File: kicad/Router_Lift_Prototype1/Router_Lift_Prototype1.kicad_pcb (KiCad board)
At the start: 2 copper layers, 150 x 100 mm, 31 parts, among them J1 Conn_01x02, J10 Conn_01x02, J11 Conn_01x04, J2 Conn_01x02, J3 Conn_01x06, J4 Conn_01x06, J5 Conn_01x06, J6 Conn_01x02, J7 Conn_01x02, J8 Conn_01x02, J9 Conn_01x02, Q1 2N7000, Q2 2N7000, U1 SH1106_Display_Module, U2 ESP32-WROOM, U3 BOOST-DRV8711

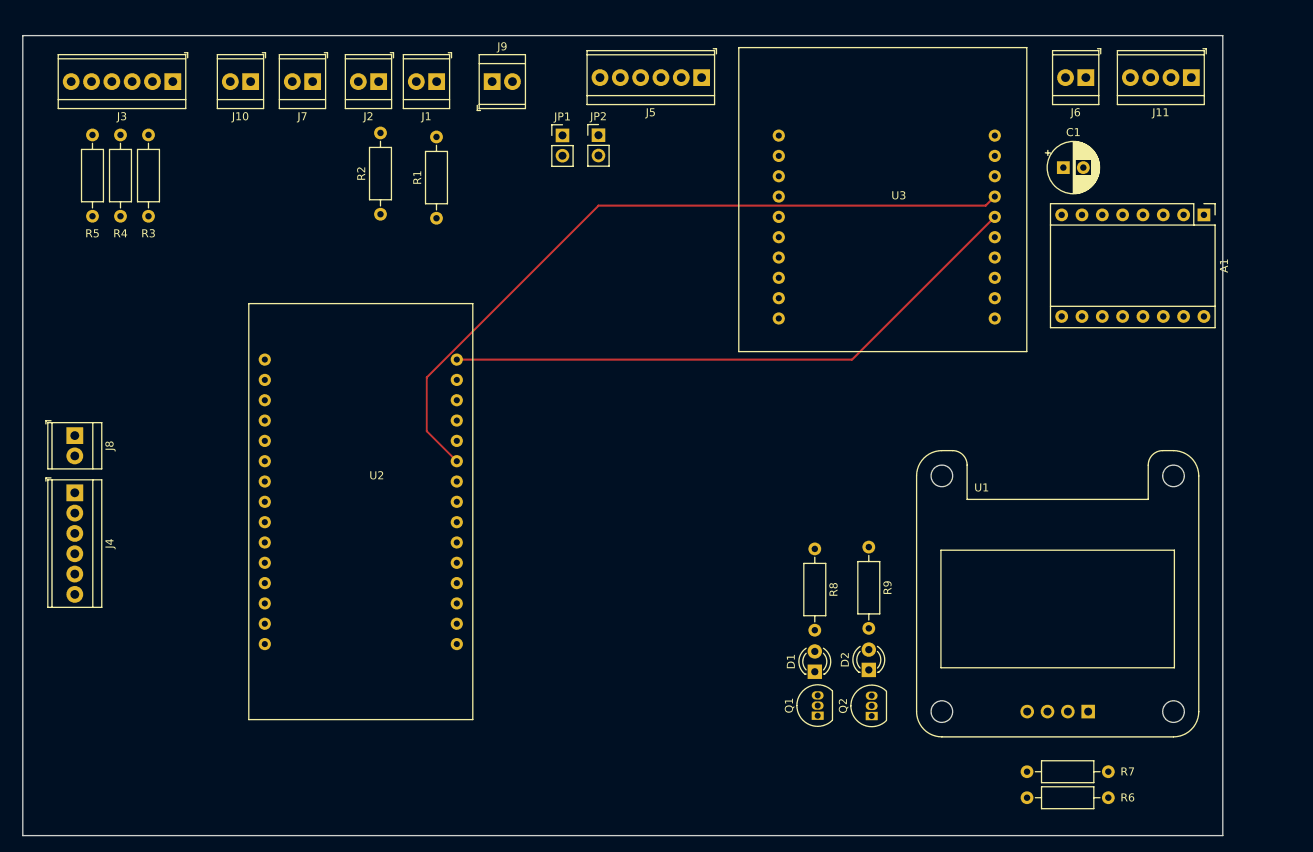
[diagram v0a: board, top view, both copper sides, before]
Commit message: Further placement
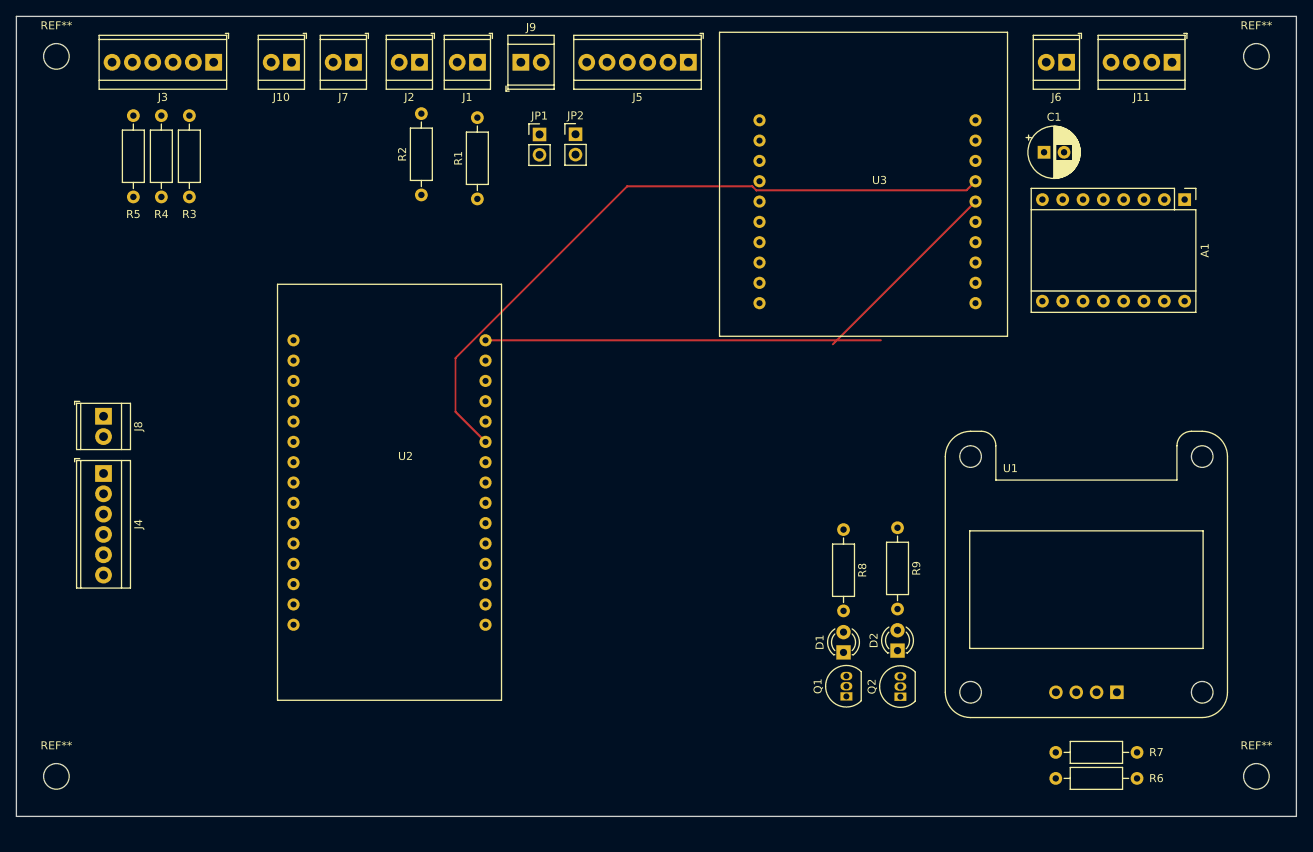
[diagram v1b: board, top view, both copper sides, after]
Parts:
- added REF**: MountingHole_3.2mm_M3_ISO7380, MountingHole:MountingHole_3.2mm_M3_ISO7380, F.Cu at (55.0, 55.0)
- added REF**: MountingHole_3.2mm_M3_ISO7380, MountingHole:MountingHole_3.2mm_M3_ISO7380, F.Cu at (205.0, 55.0)
- added REF**: MountingHole_3.2mm_M3_ISO7380, MountingHole:MountingHole_3.2mm_M3_ISO7380, F.Cu at (205.0, 145.0)
- added REF**: MountingHole_3.2mm_M3_ISO7380, MountingHole:MountingHole_3.2mm_M3_ISO7380, F.Cu at (55.0, 145.0)
- moved R4 5.65 mm to (68.1, 72.6)
- moved R5 5.65 mm to (64.6, 72.6)
- moved R1 5.65 mm to (107.6, 72.8)
- moved R2 5.65 mm to (100.6, 72.3)
- moved R3 5.65 mm to (71.6, 72.6)
- moved J1 5.65 mm to (107.6, 55.7)
- moved J10 5.65 mm to (84.4, 55.7)
- moved J2 5.65 mm to (100.4, 55.7)
- moved J3 5.65 mm to (74.7, 55.7)
- moved J7 5.65 mm to (92.1, 55.7)
- moved Q2 4.33 mm to (160.5, 135.0)
- moved J8 4.33 mm to (60.9, 100.0)
- moved U2 4.33 mm to (96.6, 109.5)
- moved J9 4.33 mm to (113.1, 55.7)
- moved J4 4.33 mm to (60.9, 107.1)
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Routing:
- net /MISO: track 92.4 -> 86.6 mm
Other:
- board size 150 x 100 mm -> 160 x 100 mm
